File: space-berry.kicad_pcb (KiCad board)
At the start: 8 copper layers, 175 parts, among them J1 USB_C_Receptacle_USB2.0, J2 RJ45_RB1-125B8G1A, J3 USB_C_Receptacle_USB2.0, Q1 SiS415DNT, Q2 TSM2302CX, U11 RTL8211F-CG, U12 K4A8G165WC-BCTD, U13 XCZU15EG-2FFVB1156E, U14 K4A8G165WC-BCTD, U15 USB3300-EZK, U16 USB3300-EZK, U17 CDCI6214RGET, U6 TLV75801PDBV, U7 TLV75801PDBV, U8 TLV75801PDBV, U9 TLV75801PDBV, X1 ECS-2520MV-xxx-xx, X2 ECS-2520MV-xxx-xx

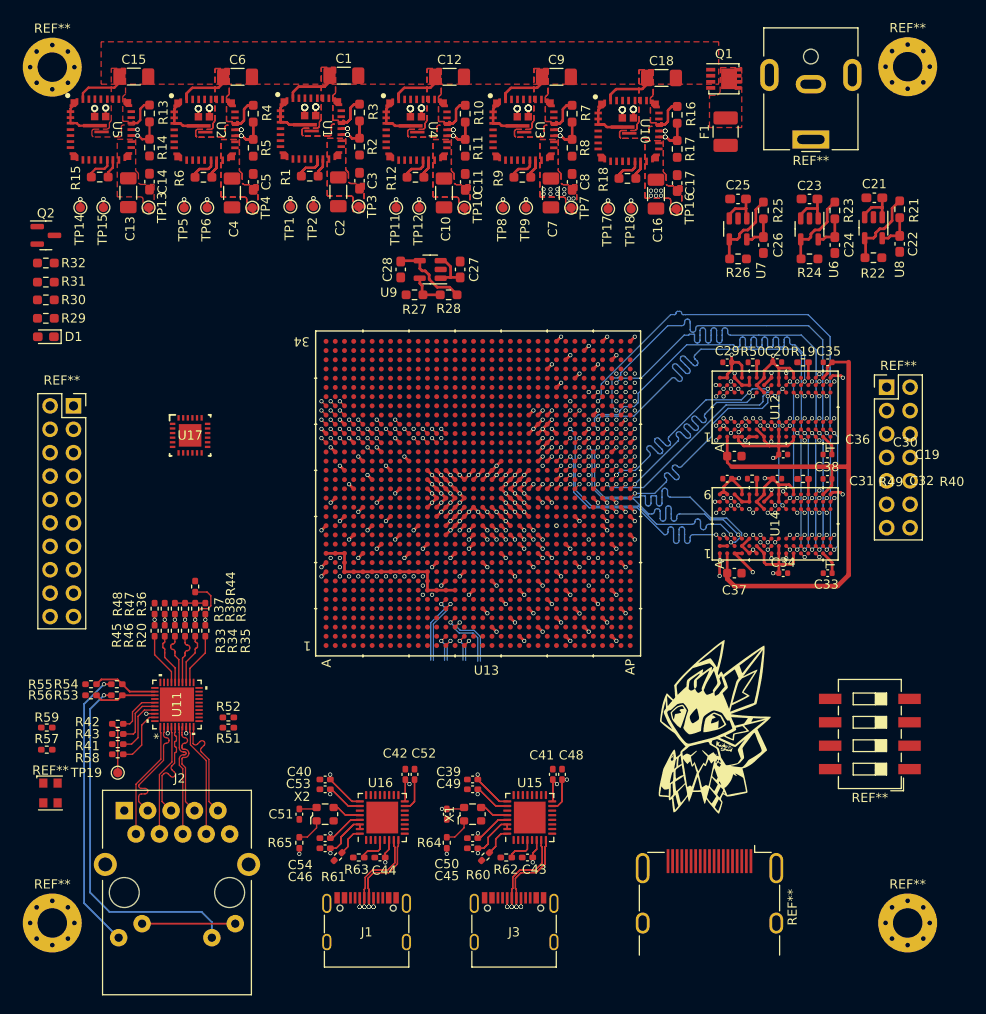
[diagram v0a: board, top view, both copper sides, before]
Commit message: stuff
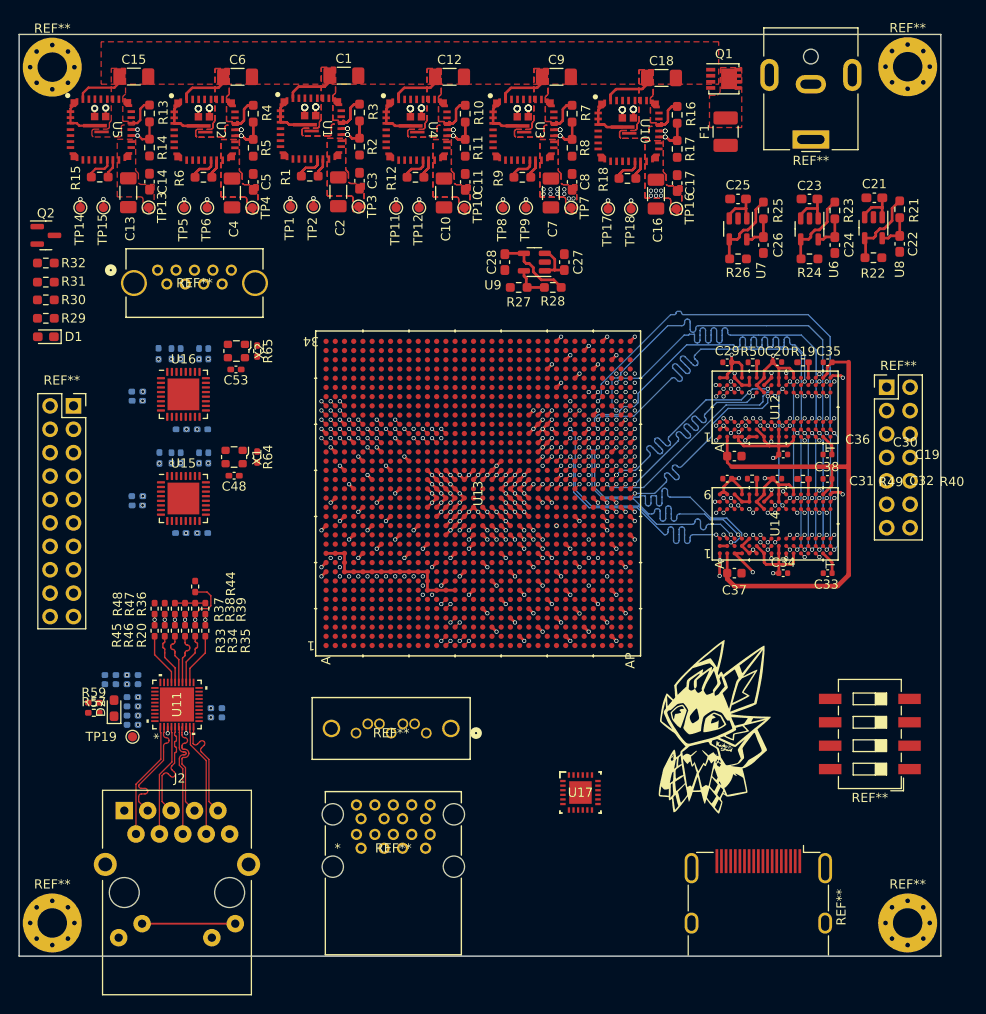
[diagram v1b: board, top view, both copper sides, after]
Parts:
- removed J1, J3: USB_C_Receptacle_USB2.0, Connector_USB:USB_C_Receptacle_G-Switch_GT-USB-7010ASV
- removed the REF** at (95.0, 126.6)
- added D2: LED, LED_SMD:LED_0603_1608Metric_Pad1.05x0.95mm_HandSolder, F.Cu at (101.9, 117.4)
- added REF**: 48406-0003_MOL, lib:48406-0003_MOL, F.Cu at (128.7, 132.6)
- added REF**: CONN9_08-0003_MOL, lib:CONN9_08-0003_MOL, F.Cu at (106.6, 69.9)
- added REF**: CONN_67800-8025_MOL, lib:CONN_67800-8025_MOL, F.Cu at (135.8, 120.1)
- C39, C40, C41, C42, C43, C44, C45, C46, C47, C49, C50, C51, C52, C54, R41, R42, R43, R51, R52, R53, R54, R55, R56, R58, R60, R61, R62, R63: moved to B.Cu
- U13: footprint lib:FFVB1156_XIL-L -> lib:FFVB1156_XIL
- moved R61 57.9 mm to (106.7, 79.0), turned to -90 degrees
- moved U17 57.4 mm to (152.5, 126.5)
- moved R62 56.0 mm to (104.4, 94.4)
- moved R63 56.0 mm to (104.4, 83.0)
- moved R60 55.9 mm to (106.8, 90.2), turned to -90 degrees
- moved C54 54.8 mm to (109.1, 79.0), turned to 90 degrees
- moved R65 53.5 mm to (117.4, 78.7)
- moved C45 53.5 mm to (108.1, 90.2), turned to 90 degrees
- moved C46 52.7 mm to (104.4, 84.0)
- moved C50 52.0 mm to (109.1, 90.2), turned to 90 degrees
- moved X2 51.2 mm to (115.2, 78.7), turned to -90 degrees
- moved C51 51.1 mm to (111.1, 79.0), turned to 90 degrees
- moved U15 51.1 mm to (109.4, 94.7), turned to 0 degrees
- moved C41 50.7 mm to (112.1, 90.2), turned to -90 degrees
- moved U16 50.7 mm to (109.4, 83.3), turned to 0 degrees
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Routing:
- net 3V3: track 74.0 -> 13.0 mm, vias 8 -> 7
- net 1V8: track 59.0 -> 4.10 mm, vias 8 -> 6
- net Net-(J2-PadL2): track 39.1 -> 0.00 mm, vias 1 -> 0
- net Net-(J2-PadL4): track 30.7 -> 0.00 mm, vias 1 -> 0
- net /USB_2_2/USB0_D-: track 23.9 -> 2.70 mm, vias 4 -> 0
- net /USB_2.0/USB0_D-: track 23.9 -> 2.70 mm, vias 4 -> 0
- net /USB_2.0/USB0_D+: track 23.9 -> 2.67 mm, vias 4 -> 0
- net /USB_2_2/USB0_D+: track 23.9 -> 2.67 mm, vias 4 -> 0
- net ETH_LED_G: track 7.09 -> 0.00 mm, vias 0 -> 1
- net DP_L2_TX-: track 7.58 -> 0.71 mm
- net DP_L2_TX+: track 7.58 -> 0.71 mm
- net ETH_LED_Y: track 6.76 -> 0.00 mm, vias 0 -> 1
- net Net-(U16-VBUS): track 6.56 -> 0.00 mm, vias 0 -> 1
- net Net-(U15-VBUS): track 6.56 -> 0.00 mm, vias 0 -> 1
- net Net-(U16-RBIAS): track 6.53 -> 0.00 mm, vias 0 -> 1
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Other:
- board outline added: 100 x 100 mm
